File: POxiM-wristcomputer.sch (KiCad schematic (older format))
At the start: 8 parts, among them J1 Power in

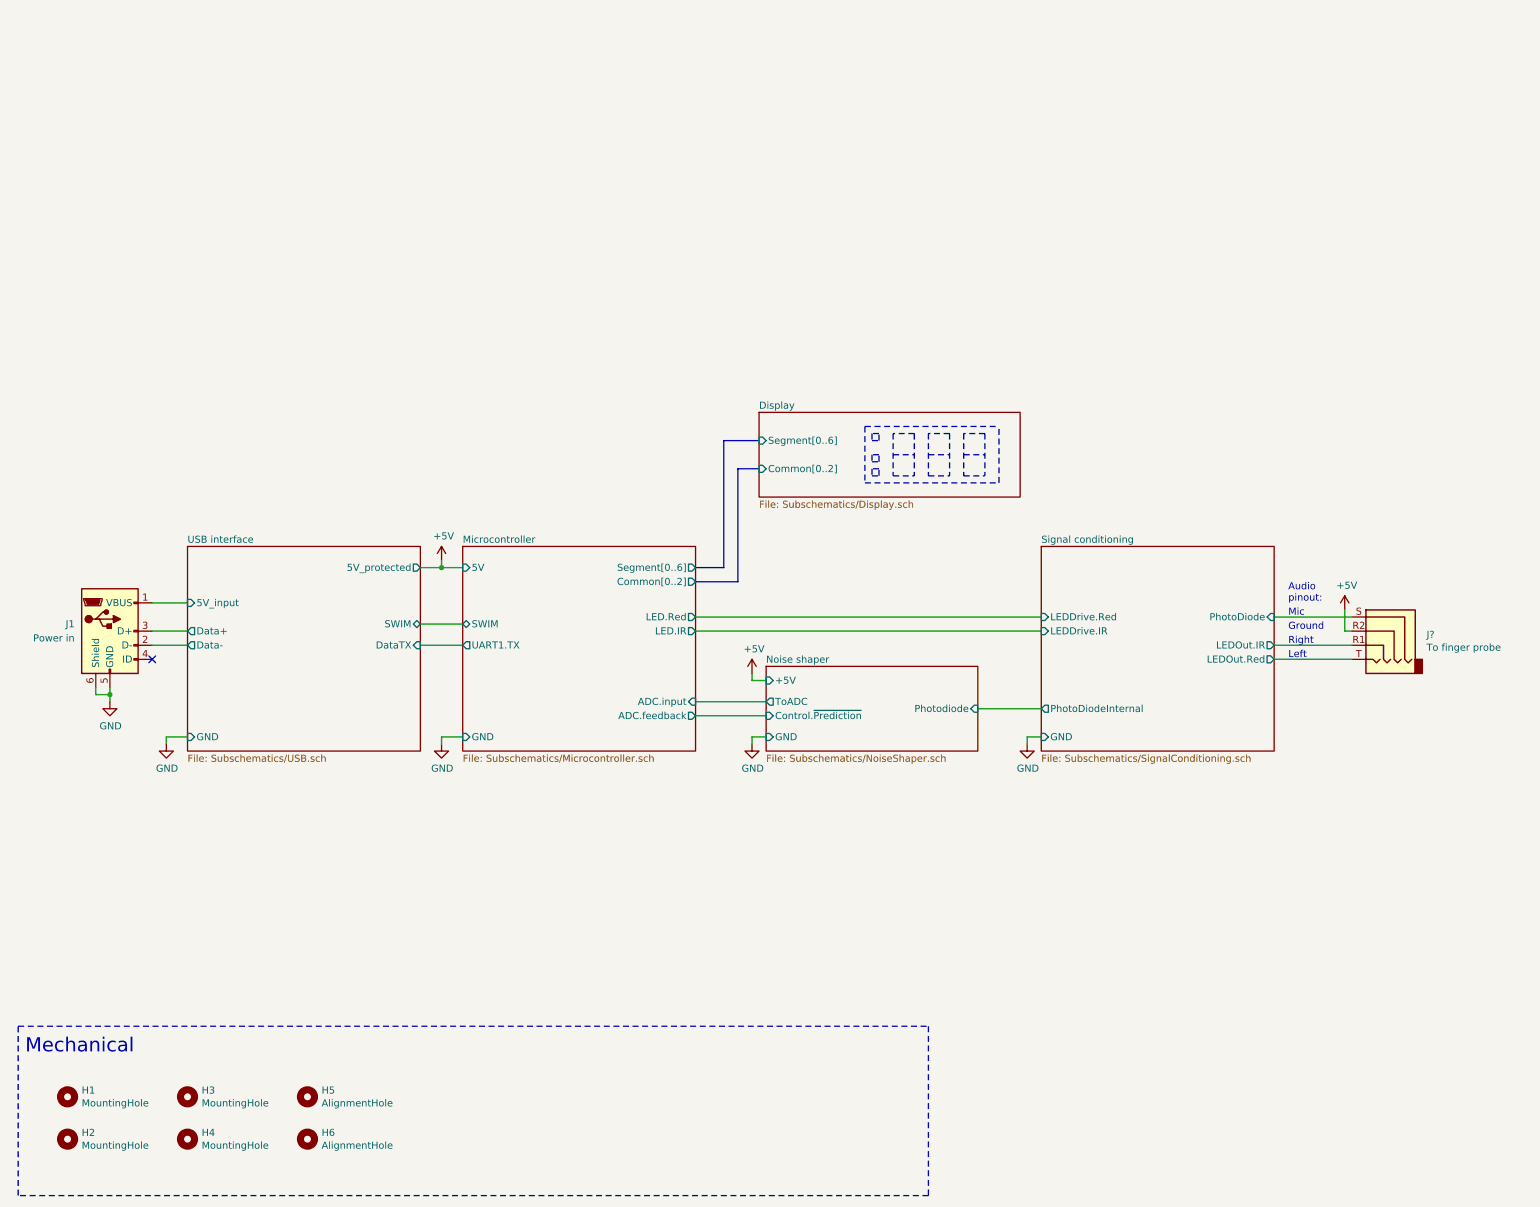
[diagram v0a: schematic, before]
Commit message: Cleanup most of schematic
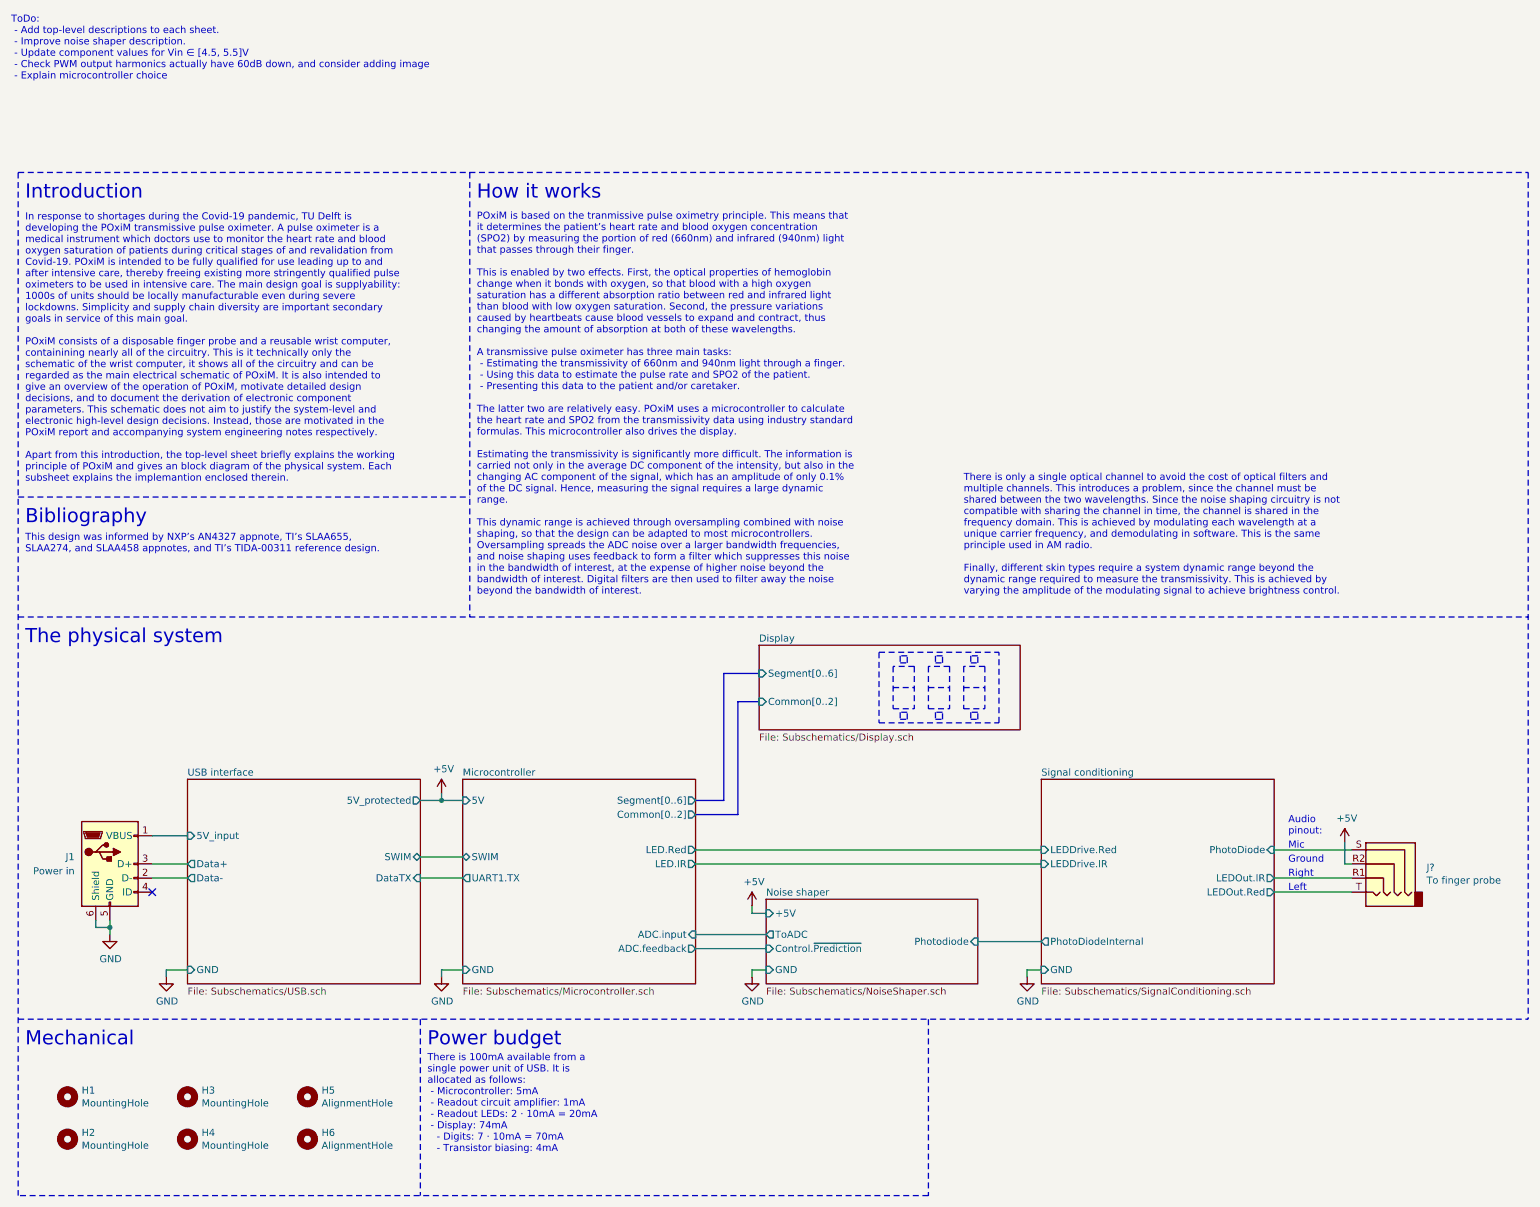
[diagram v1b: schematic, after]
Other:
- note added: "Bibliography"
- note added: "How it works"
- note added: "In response to shortages during the Covid-19 pandemic, TU Delft is \ndeveloping the POxiM transmissive pulse oximeter. A pulse oximeter is a \nmedical instrument which doctors use to monitor the heart rate and blood \noxygen saturation of patients during critical stages of and revalidation from \nCovid-19. POxiM is intended to be fully qualified for use leading up to and \nafter intensive care, t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"
- note added: "Introduction"
- note added: "POxiM is based on the tranmissive pulse oximetry principle. This means that \nit determines the patient’s heart rate and blood oxygen concentration \n(SPO2) by measuring the portion of red (660nm) and infrared (940nm) light \nthat passes through their finger.\n\nThis is enabled by two effects. First, the optical properties of hemoglobin \nchange when it bonds with oxygen, so that blood with a hig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"
- note added: "Power budget"
- note added: "The physical system"
- note added: "There is 100mA available from a\nsingle power unit of USB. It is\nallocated as follows:\n - Microcontroller: 5mA\n - Readout circuit amplifier: 1mA\n - Readout LEDs: 2 · 10mA = 20mA\n - Display: 74mA\n - Digits: 7 · 10mA = 70mA\n - Transistor biasing: 4mA"
- note added: "There is only a single optical channel to avoid the cost of optical filters and \nmultiple channels. This introduces a problem, since the channel must be \nshared between the two wavelengths. Since the noise shaping circuitry is not \ncompatible with sharing the channel in time, the channel is shared in the \nfrequency domain. This is achieved by modulating each wavelength at a \nunique carrier f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"
- note added: "This design was informed by NXP’s AN4327 appnote, TI’s SLAA655, \nSLAA274, and SLAA458 appnotes, and TI’s TIDA-00311 reference design."
- note added: "ToDo:\n - Add top-level descriptions to each sheet.\n - Improve noise shaper description.\n - Update component values for Vin ∈ [4.5, 5.5]V\n - Check PWM output harmonics actually have 60dB down, and consider adding image\n - Explain microcontroller choice"
- moved on the sheet: J1, J?
